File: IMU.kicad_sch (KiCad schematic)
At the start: 5 parts, among them J3 5033981892, U1 ICM-42688-P

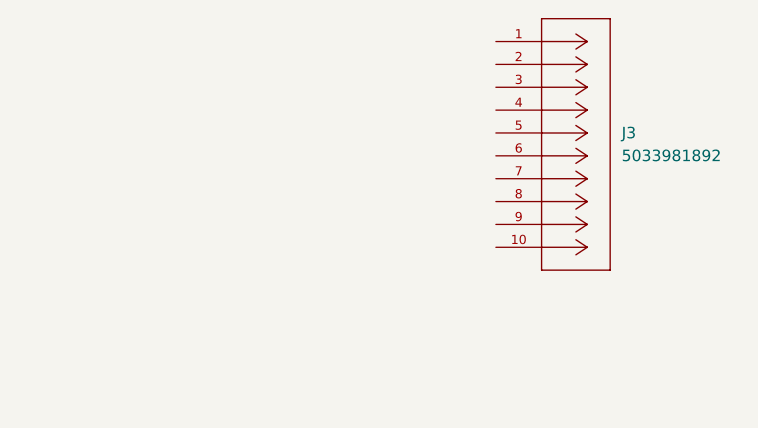
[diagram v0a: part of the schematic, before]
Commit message: filter for CAN
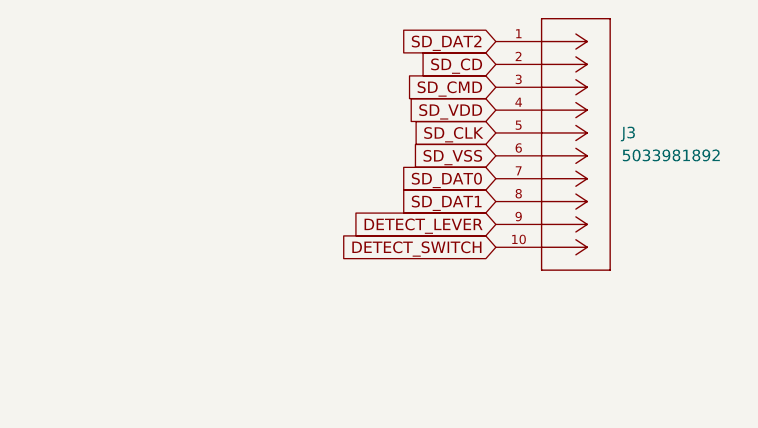
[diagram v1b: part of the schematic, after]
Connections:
- net SD_DAT2: now reaches J3.1
- net DETECT_SWITCH: now reaches J3.10
- net SD_CD: now reaches J3.2
- net SD_CMD: now reaches J3.3
- net SD_VDD: now reaches J3.4
- net SD_CLK: now reaches J3.5
- net SD_VSS: now reaches J3.6
- net SD_DAT0: now reaches J3.7
- net SD_DAT1: now reaches J3.8
- net DETECT_LEVER: now reaches J3.9
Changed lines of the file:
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@@
+		)
+	)
+	(global_label "SD_DAT0"
+		(shape input)
+		(at 243.84 78.74 180)
+		(fields_autoplaced yes)
+		(effects
+			(font
+				(size 1.27 1.27)
+			)
+			(justify right)
+		)
+		(property "Intersheetrefs" "${INTERSHEET_REFS}"
+			(at 232.872 78.74 0)
+			(effects
+				(font
+					(size 1.27 1.27)
+				)
+				(justify right)
+				(hide yes)
+			)
+		)
+	)
+	(global_label "SD_CLK"
+		(shape input)
+		(at 243.84 73.66 180)
+		(fields_autoplaced yes)
+		(effects
+			(font
+				(size 1.27 1.27)
+			)
+			(justify right)
+		)
+		(property "Intersheetrefs" "${INTERSHEET_REFS}"
+			(at 233.8396 73.66 0)
+			(effects
+				(font
+					(size 1.27 1.27)
+				)
+				(justify right)
+				(hide yes)
+			)
 		)
 	)
@@
 		)
 	)
+	(global_label "SD_CD"
+		(shape input)
+		(at 243.84 66.04 180)
+		(fields_autoplaced yes)
+		(effects
+			(font
+				(size 1.27 1.27)
+			)
+			(justify right)
+		)
+		(property "Intersheetrefs" "${INTERSHEET_REFS}"
+			(at 234.8677 66.04 0)
+			(effects
+				(font
+					(size 1.27 1.27)
+				)
+				(justify right)
+				(hide yes)
+			)
+		)
+	)
 	(global_label "IMU_CS"
 		(shape input)
@@
 		)
 	)
+	(global_label "DETECT_LEVER"
+		(shape input)
+		(at 243.84 83.82 180)
+		(fields_autoplaced yes)
+		(effects
+			(font
+				(size 1.27 1.27)
+			)
+			(justify right)
+		)
+		(property "Intersheetrefs" "${INTERSHEET_REFS}"
+			(at 227.4293 83.82 0)
+			(effects
+				(font
+					(size 1.27 1.27)
+				)
+				(justify right)
+				(hide yes)
+			)
+		)
+	)
+	(global_label "SD_DAT1"
+		(shape input)
+		(at 243.84 81.28 180)
+		(fields_autoplaced yes)
+		(effects
+			(font
+				(size 1.27 1.27)
+			)
+			(justify right)
+		)
+		(property "Intersheetrefs" "${INTERSHEET_REFS}"
+			(at 232.872 81.28 0)
+			(effects
+				(font
+					(size 1.27 1.27)
+				)
+				(justify right)
+				(hide yes)
+			)
+		)
+	)
+	(global_label "SD_VSS"
+		(shape input)
+		(at 243.84 76.2 180)
+		(fields_autoplaced yes)
+		(effects
+			(font
+				(size 1.27 1.27)
+			)
+			(justify right)
+		)
+		(property "Intersheetrefs" "${INTERSHEET_REFS}"
+			(at 233.9001 76.2 0)
+			(effects
+				(font
+					(size 1.27 1.27)
+				)
+				(justify right)
+				(hide yes)
+			)
+		)
+	)
 	(global_label "SCK"
 		(shape input)
@@
 		)
 	)
+	(global_label "DETECT_SWITCH"
+		(shape input)
+		(at 243.84 86.36 180)
+		(fields_autoplaced yes)
+		(effects
+			(font
+				(size 1.27 1.27)
+			)
+			(justify right)
+		)
+		(property "Intersheetrefs" "${INTERSHEET_REFS}"
+			(at 226.2802 86.36 0)
+			(effects
+				(font
+					(size 1.27 1.27)
+				)
+				(justify right)
+				(hide yes)
+			)
+		)
+	)
+	(global_label "SD_VDD"
+		(shape input)
+		(at 243.84 71.12 180)
+		(fields_autoplaced yes)
+		(effects
+			(font
+				(size 1.27 1.27)
+			)
+			(justify right)
+		)
+		(property "Intersheetrefs" "${INTERSHEET_REFS}"
+			(at 233.7791 71.12 0)
+			(effects
+				(font
+					(size 1.27 1.27)
+				)
+				(justify right)
+				(hide yes)
+			)
+		)
+	)
 	(global_label "SDI"
 		(shape input)
@@
 			(effects
 				(font
+					(size 1.27 1.27)
+				)
+				(justify right)
+				(hide yes)
+			)
+		)
+	)
+	(global_label "SD_DAT2"
+		(shape input)
+		(at 243.84 63.5 180)
+		(fields_autoplaced yes)
+		(effects
+			(font
+				(size 1.27 1.27)
+			)
+			(justify right)
+		)
+		(property "Intersheetrefs" "${INTERSHEET_REFS}"
+			(at 232.872 63.5 0)
+			(effects
+				(font
+					(size 1.27 1.27)
+				)
+				(justify right)
+				(hide yes)
+			)
+		)
+	)
+	(global_label "SD_CMD"
+		(shape input)
+		(at 243.84 68.58 180)
+		(fields_autoplaced yes)
+		(effects
+			(font
+				(size 1.27 1.27)
+			)
+			(justify right)
+		)
+		(property "Intersheetrefs" "${INTERSHEET_REFS}"
+			(at 233.4163 68.58 0)
+			(effects
+				(font

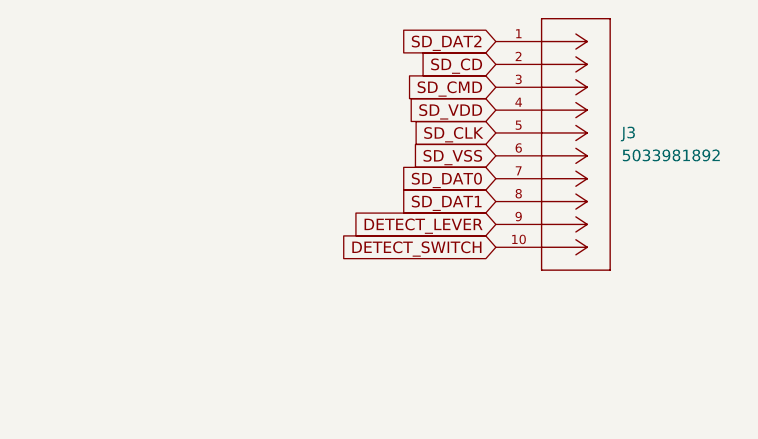
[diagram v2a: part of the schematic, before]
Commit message: new
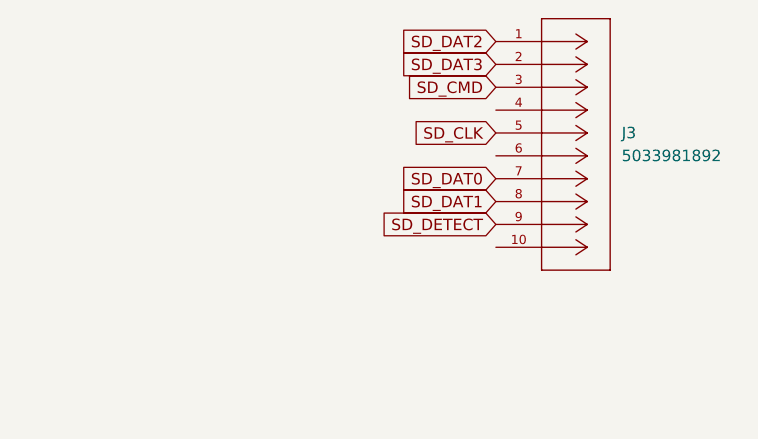
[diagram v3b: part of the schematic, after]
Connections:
- net DETECT_LEVER renamed SD_DETECT
- net DETECT_SWITCH: no longer names the net of J3.10
- net SD_CD renamed SD_DAT3
- net SD_VDD: no longer names the net of J3.4
- net SD_VSS: no longer names the net of J3.6
